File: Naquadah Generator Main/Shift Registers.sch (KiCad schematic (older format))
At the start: 4 parts, among them U2 74HC595, U3 74HC595

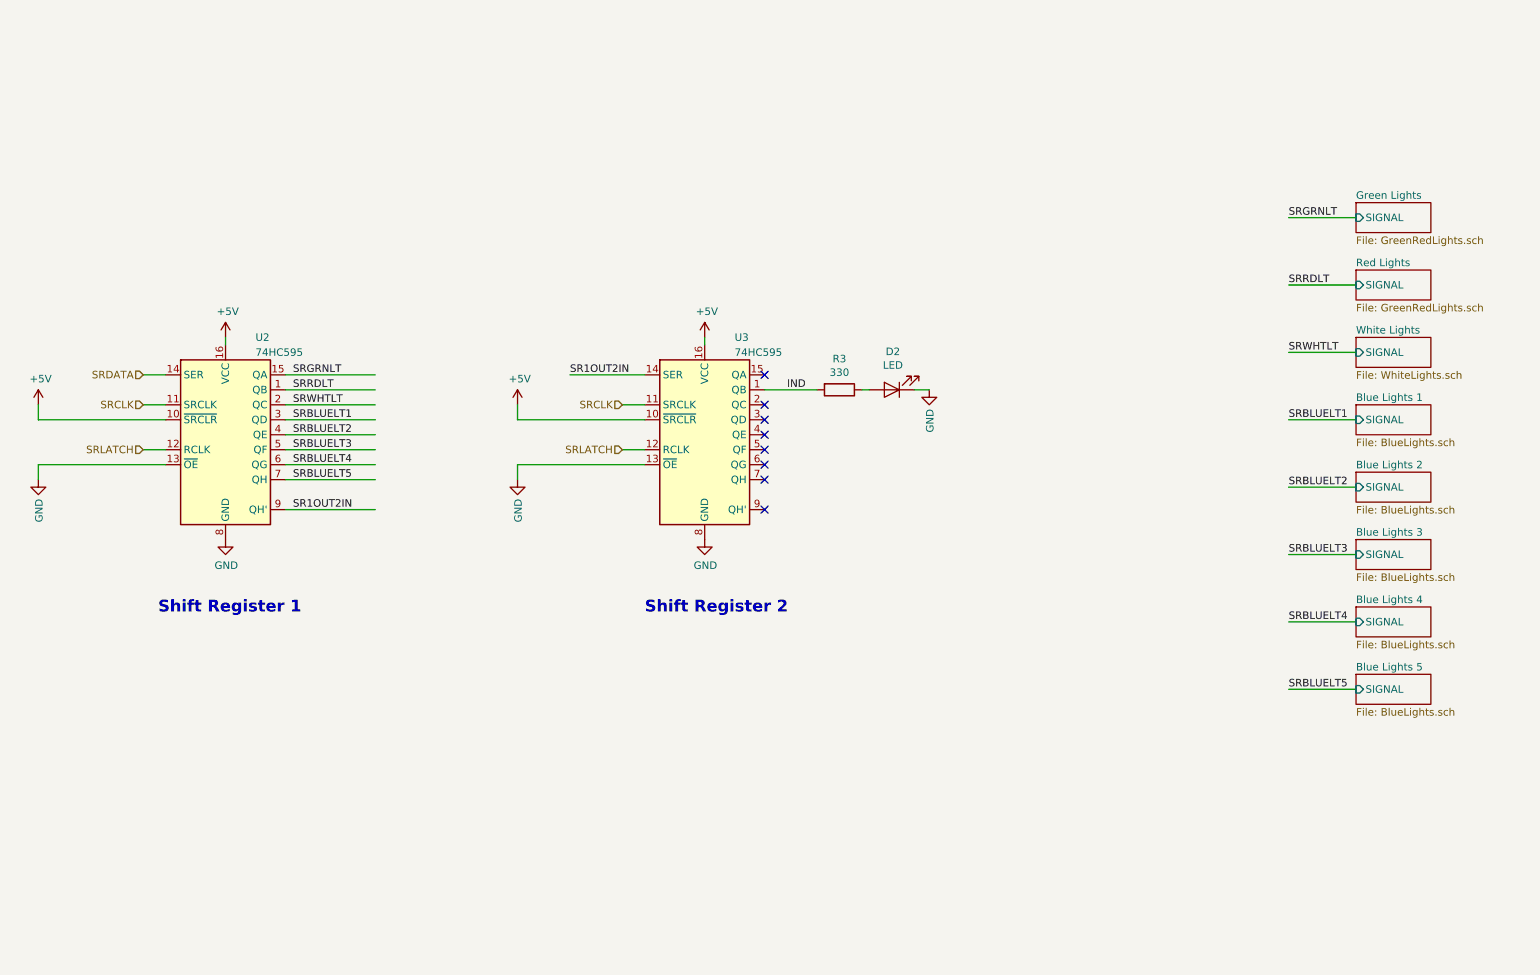
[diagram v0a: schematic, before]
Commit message: Resize to correct for scale
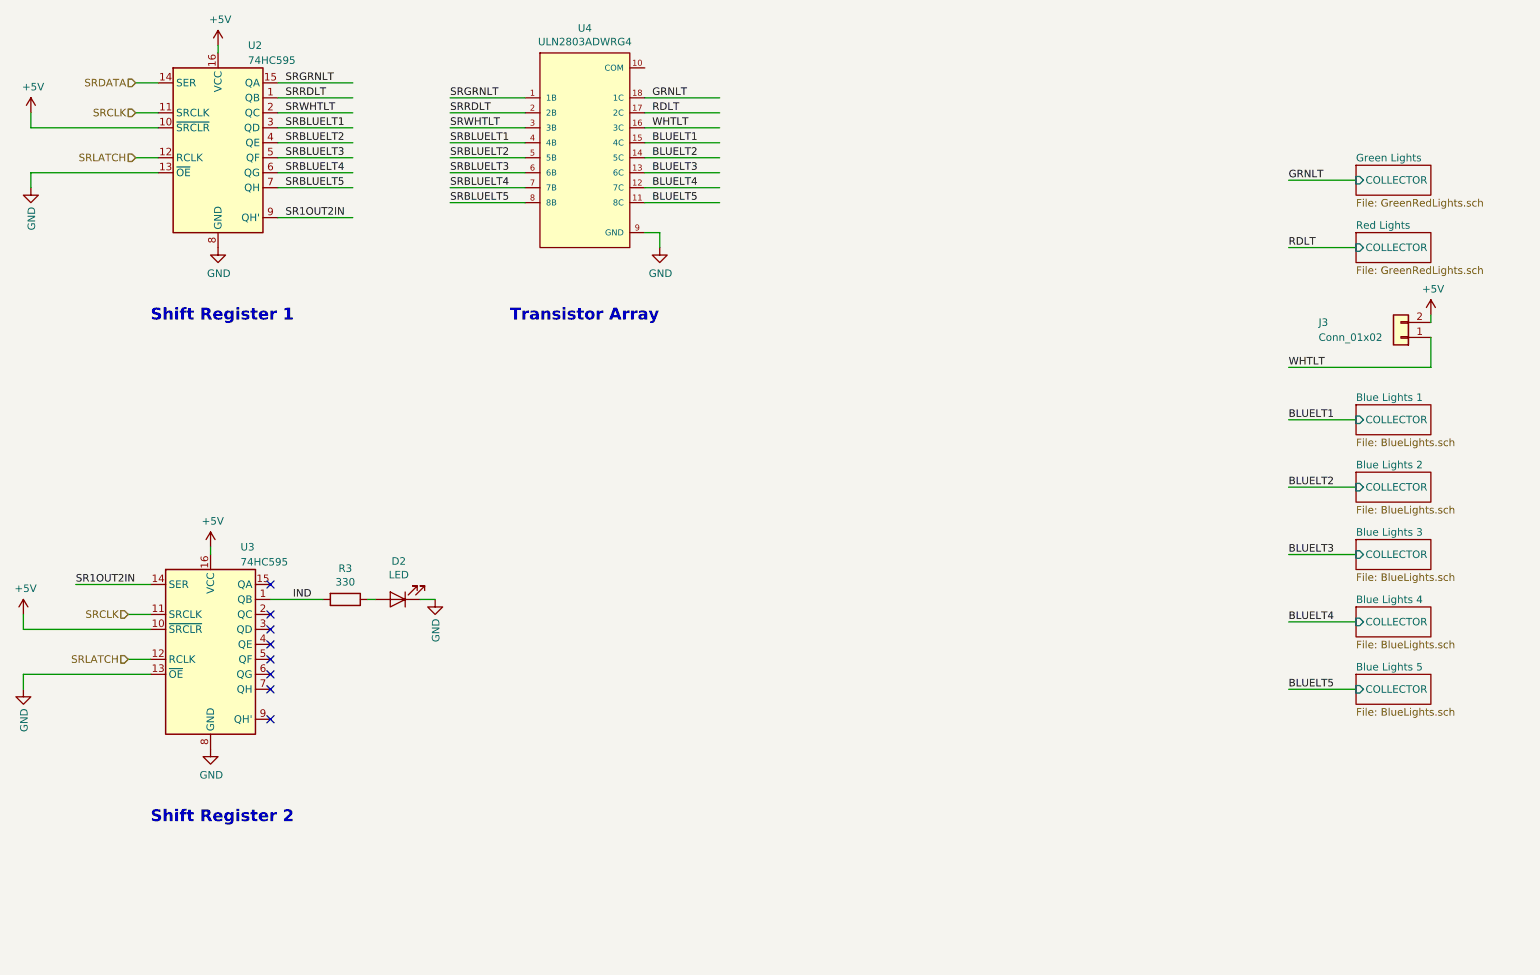
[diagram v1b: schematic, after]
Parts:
- added J3: Conn_01x02, Connector_Wire:SolderWirePad_1x02_P3.81mm_Drill1.2mm, symbol Connector_Generic:Conn_01x02
- added U4: ULN2803ADWRG4, Naquadah_Generator:SOIC127P1030X265-18N, symbol Naquadah_Generator:ULN2803ADWRG4
- U2, U3: footprint Package_DIP:DIP-16_W7.62mm -> Naquadah_Generator:SOIC-16_3.9x9.9mm_P1.27mm_Hand_Solder; Digikey Part No. (none) -> 296-14857-1-ND; Manufacturer Name (none) -> Texas Instruments; Manufacturer Part No. (none) -> SN74HC595DR
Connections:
- net labels added: BLUELT1, BLUELT2, BLUELT3, BLUELT4, BLUELT5, GRNLT, RDLT, WHTLT
- wire segments 36 -> 56
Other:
- note added: "Transistor Array"
- moved on the sheet: D2, R3, U2, U3

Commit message: Updates
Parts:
- U2, U3, U4: Description (none) -> Texas Instruments
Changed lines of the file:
@@
 $Descr A4 11693 8268
 encoding utf-8
-Sheet 3 10
+Sheet 3 11
 Title ""
 Date ""
@@
 F 5 "Texas Instruments" H 2400 1950 50  0001 C CNN "Manufacturer Name"
 F 6 "SN74HC595DR" H 2400 1950 50  0001 C CNN "Manufacturer Part No."
+F 7 "Texas Instruments" H 2400 1950 50  0001 C CNN "Description"
 	1    2400 1950
 	1    0    0    -1
@@
 F 5 "Texas Instruments" H 4850 1950 50  0001 C CNN "Manufacturer Name"
 F 6 "ULN2803ADWR" H 4850 1950 50  0001 C CNN "Manufacturer Part No."
+F 7 "Texas Instruments" H 4850 1950 50  0001 C CNN "Description"
 	1    4850 1950
 	1    0    0    -1
@@
 F 5 "Texas Instruments" H 2350 5300 50  0001 C CNN "Manufacturer Name"
 F 6 "SN74HC595DR" H 2350 5300 50  0001 C CNN "Manufacturer Part No."
+F 7 "Texas Instruments" H 2350 5300 50  0001 C CNN "Description"
 	1    2350 5300
 	1    0    0    -1

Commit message: Adding Power Daughter Board
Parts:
- U2, U3: Digikey Part No. 296-14857-1-ND -> (none); Source (none) -> Digikey; Source Part No. (none) -> 296-14857-1-ND
- U4: Digikey Part No. 296-15777-1-ND -> (none); Source (none) -> Digikey; Source Part No. (none) -> 296-15777-1-ND
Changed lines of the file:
@@
 F 2 "Naquadah_Generator:SOIC-16_3.9x9.9mm_P1.27mm_Hand_Solder" H 2400 1950 50  0001 C CNN
 F 3 "http://www.ti.com/lit/ds/symlink/sn74hc595.pdf?HQS=TI-null-null-digikeymode-df-pf-null-wwe&ts=1590028307018" H 2400 1950 50  0001 C CNN
-F 4 "296-14857-1-ND" H 2400 1950 50  0001 C CNN "Digikey Part No."
+F 4 "296-14857-1-ND" H 2400 1950 50  0001 C CNN "Source Part No."
 F 5 "Texas Instruments" H 2400 1950 50  0001 C CNN "Manufacturer Name"
 F 6 "SN74HC595DR" H 2400 1950 50  0001 C CNN "Manufacturer Part No."
 F 7 "Texas Instruments" H 2400 1950 50  0001 C CNN "Description"
+F 8 "Digikey" H 2400 1950 50  0001 C CNN "Source"
 	1    2400 1950
 	1    0    0    -1
@@
 F 2 "Naquadah_Generator:SOIC127P1030X265-18N" H 4550 1050 50  0001 L BNN
 F 3 "http://www.ti.com/lit/ds/symlink/uln2803a.pdf?HQS=TI-null-null-digikeymode-df-pf-null-wwe&ts=1590002980089" H 4850 1950 50  0001 L BNN
-F 4 "296-15777-1-ND" H 4850 1950 50  0001 C CNN "Digikey Part No."
+F 4 "296-15777-1-ND" H 4850 1950 50  0001 C CNN "Source Part No."
 F 5 "Texas Instruments" H 4850 1950 50  0001 C CNN "Manufacturer Name"
 F 6 "ULN2803ADWR" H 4850 1950 50  0001 C CNN "Manufacturer Part No."
 F 7 "Texas Instruments" H 4850 1950 50  0001 C CNN "Description"
+F 8 "Digikey" H 4850 1950 50  0001 C CNN "Source"
 	1    4850 1950
 	1    0    0    -1
@@
 F 2 "Naquadah_Generator:SOIC-16_3.9x9.9mm_P1.27mm_Hand_Solder" H 2350 5300 50  0001 C CNN
 F 3 "http://www.ti.com/lit/ds/symlink/sn74hc595.pdf?HQS=TI-null-null-digikeymode-df-pf-null-wwe&ts=1590028307018" H 2350 5300 50  0001 C CNN
-F 4 "296-14857-1-ND" H 2350 5300 50  0001 C CNN "Digikey Part No."
+F 4 "296-14857-1-ND" H 2350 5300 50  0001 C CNN "Source Part No."
 F 5 "Texas Instruments" H 2350 5300 50  0001 C CNN "Manufacturer Name"
 F 6 "SN74HC595DR" H 2350 5300 50  0001 C CNN "Manufacturer Part No."
 F 7 "Texas Instruments" H 2350 5300 50  0001 C CNN "Description"
+F 8 "Digikey" H 2350 5300 50  0001 C CNN "Source"
 	1    2350 5300
 	1    0    0    -1

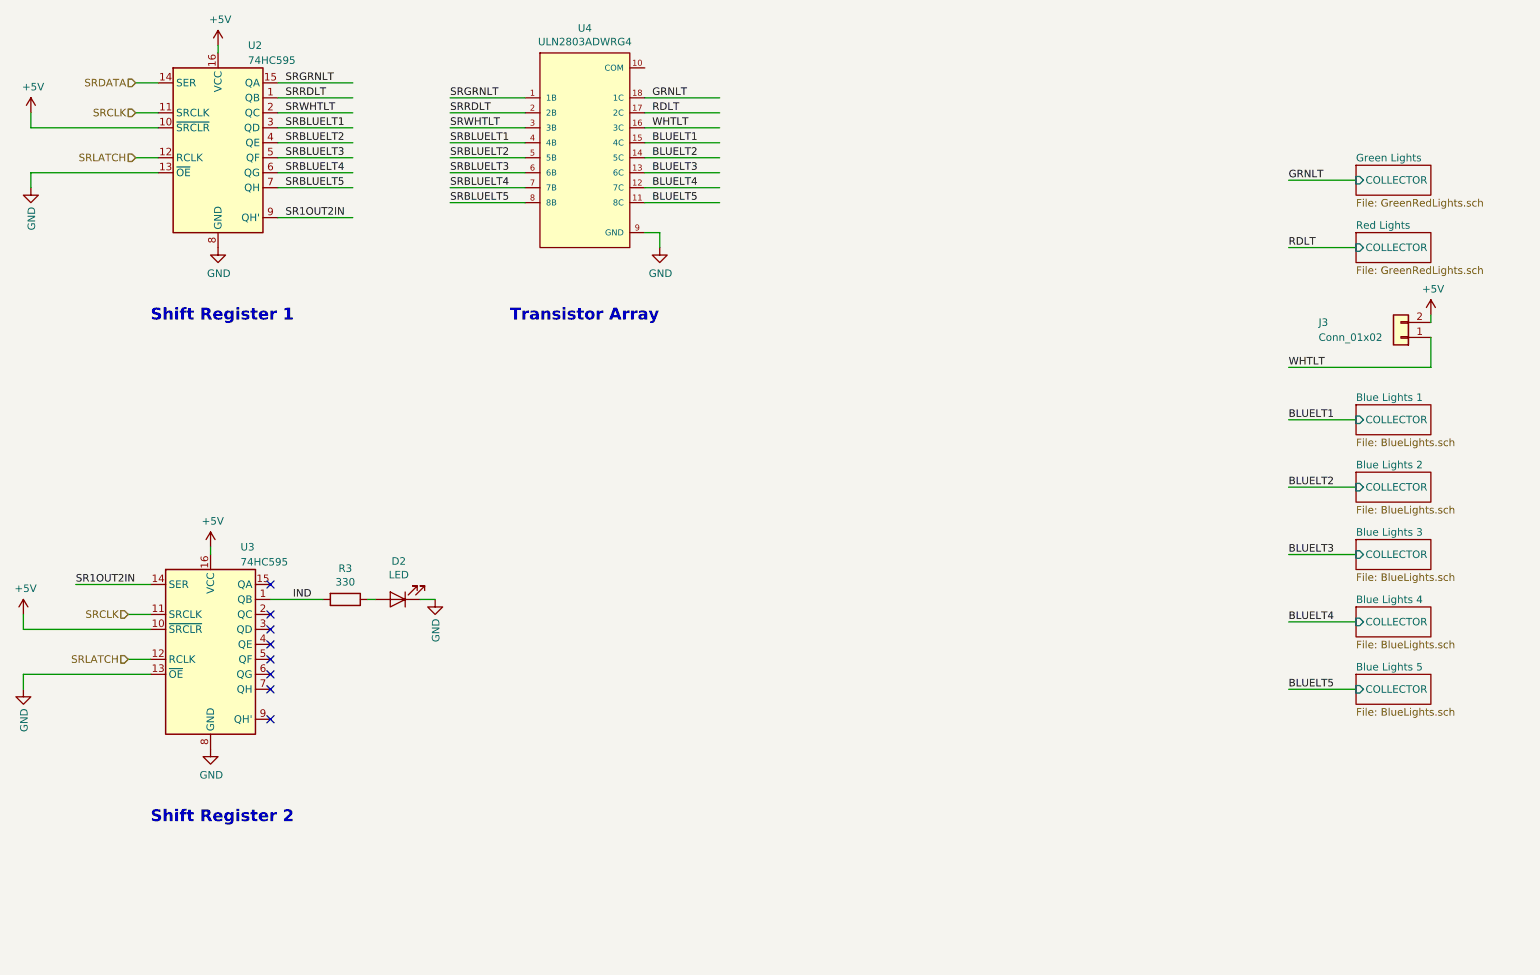
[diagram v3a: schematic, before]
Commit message: Updates
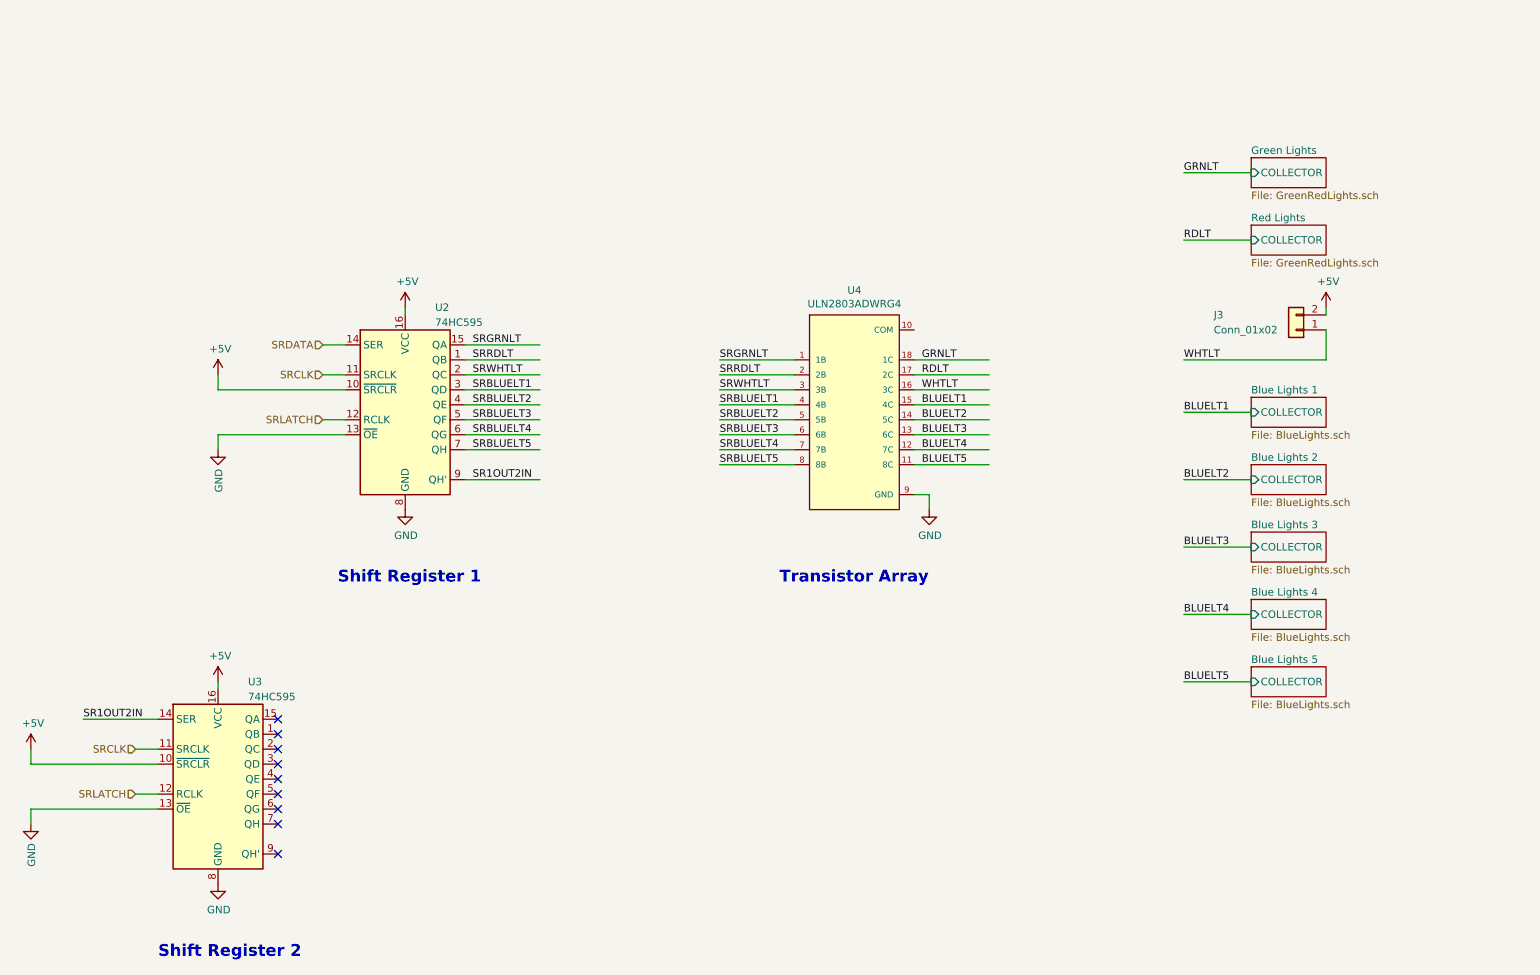
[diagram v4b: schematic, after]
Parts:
- removed D2: LED, LED_THT:LED_D5.0mm, symbol Frequently_Used:LED
- removed R3: 330, Frequently_Used:0805_2012Metric_HandSolder, symbol Frequently_Used:R
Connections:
- net labels removed: IND
- wire segments 56 -> 53
- no-connect marks 8 -> 9
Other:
- moved on the sheet: J3, U2, U3, U4

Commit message: Updates
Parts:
- U4: Description Texas Instruments -> Bipolar (BJT) Transistor Array 8 NPN Darlington 50V 500mA S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
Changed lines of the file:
@@
 F 5 "Texas Instruments" H 6650 3700 50  0001 C CNN "Manufacturer Name"
 F 6 "ULN2803ADWR" H 6650 3700 50  0001 C CNN "Manufacturer Part No."
-F 7 "Texas Instruments" H 6650 3700 50  0001 C CNN "Description"
+F 7 "Bipolar (BJT) Transistor Array 8 NPN Darlington 50V 500mA Surface Mount 18-SOIC" H 6650 3700 50  0001 C CNN "Description"
 F 8 "Digikey" H 6650 3700 50  0001 C CNN "Source"
 	1    6650 3700
